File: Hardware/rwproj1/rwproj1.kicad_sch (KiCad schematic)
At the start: 4 parts, among them J1 Conn_01x02, SW1 SW_Push

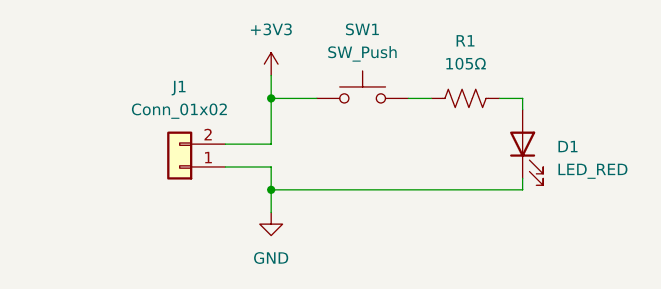
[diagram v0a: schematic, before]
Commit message: HW P1
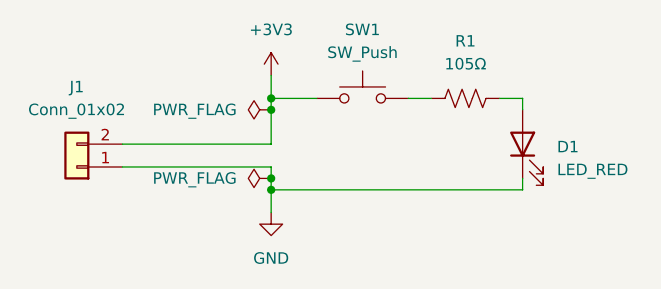
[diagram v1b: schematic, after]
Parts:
- J1: MPN (none) -> 022272021; Notes (none) -> May change to blue
- SW1: MPN (none) -> 1825910-6
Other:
- moved on the sheet: J1
